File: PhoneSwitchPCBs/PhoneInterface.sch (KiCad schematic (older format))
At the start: 37 parts

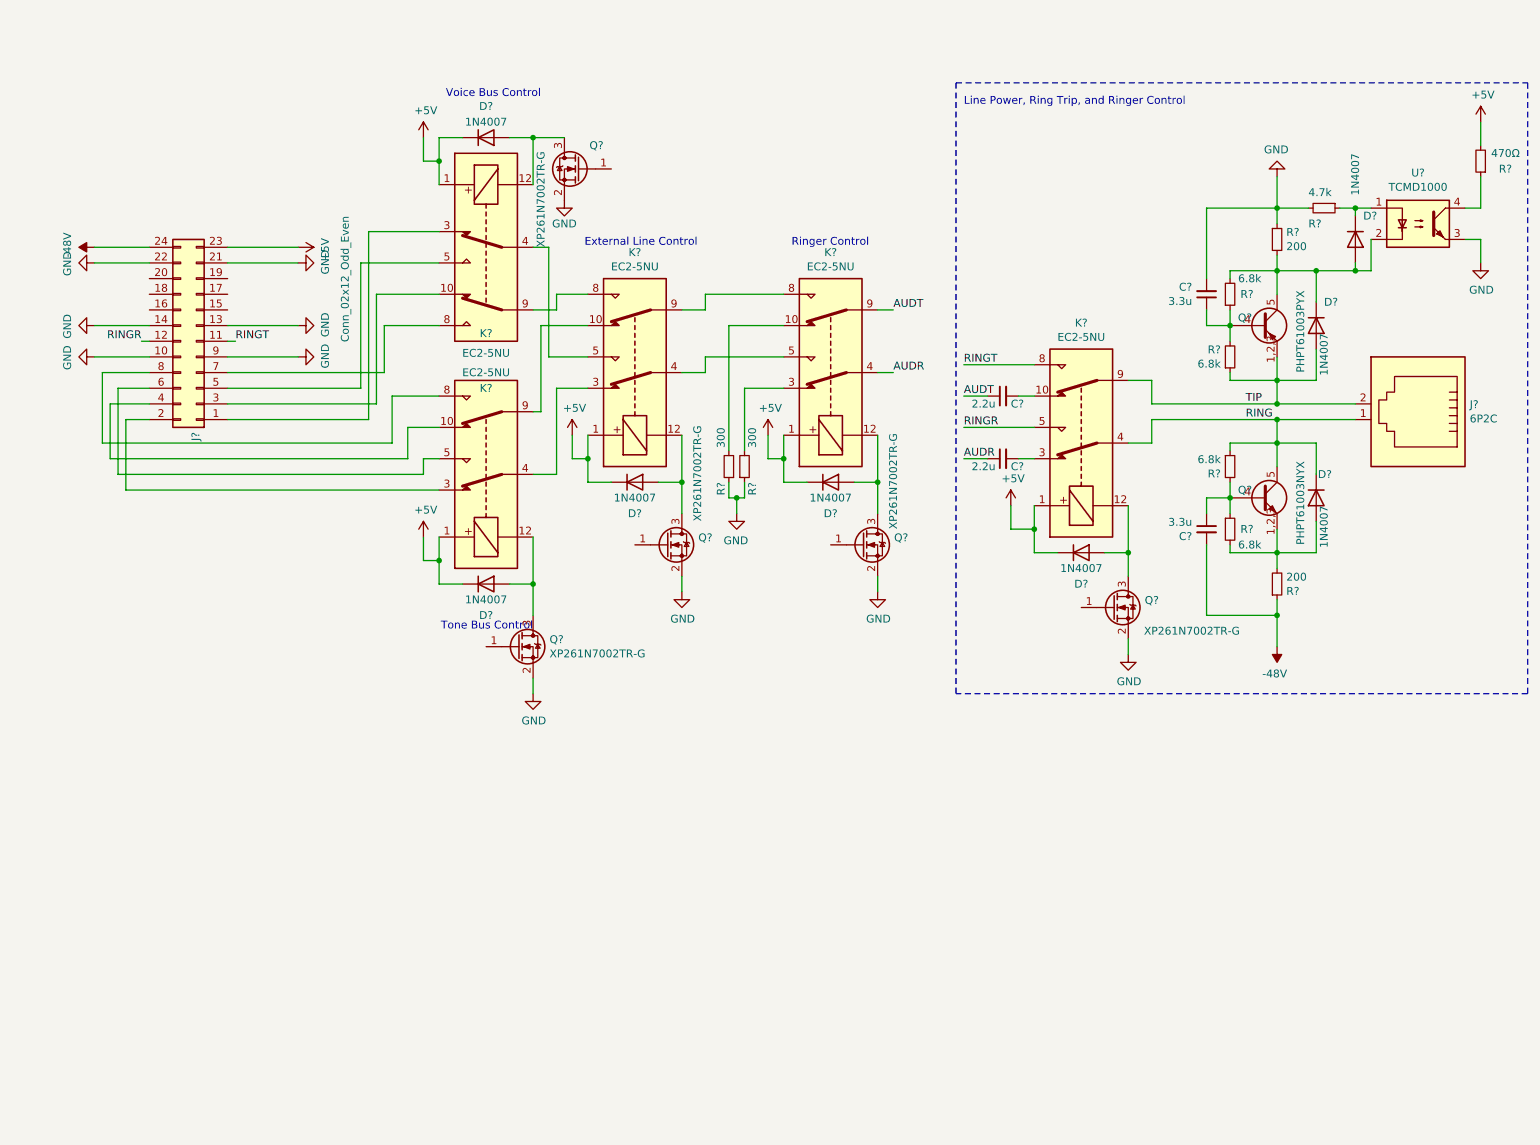
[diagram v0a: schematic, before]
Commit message: Continued work on schematic
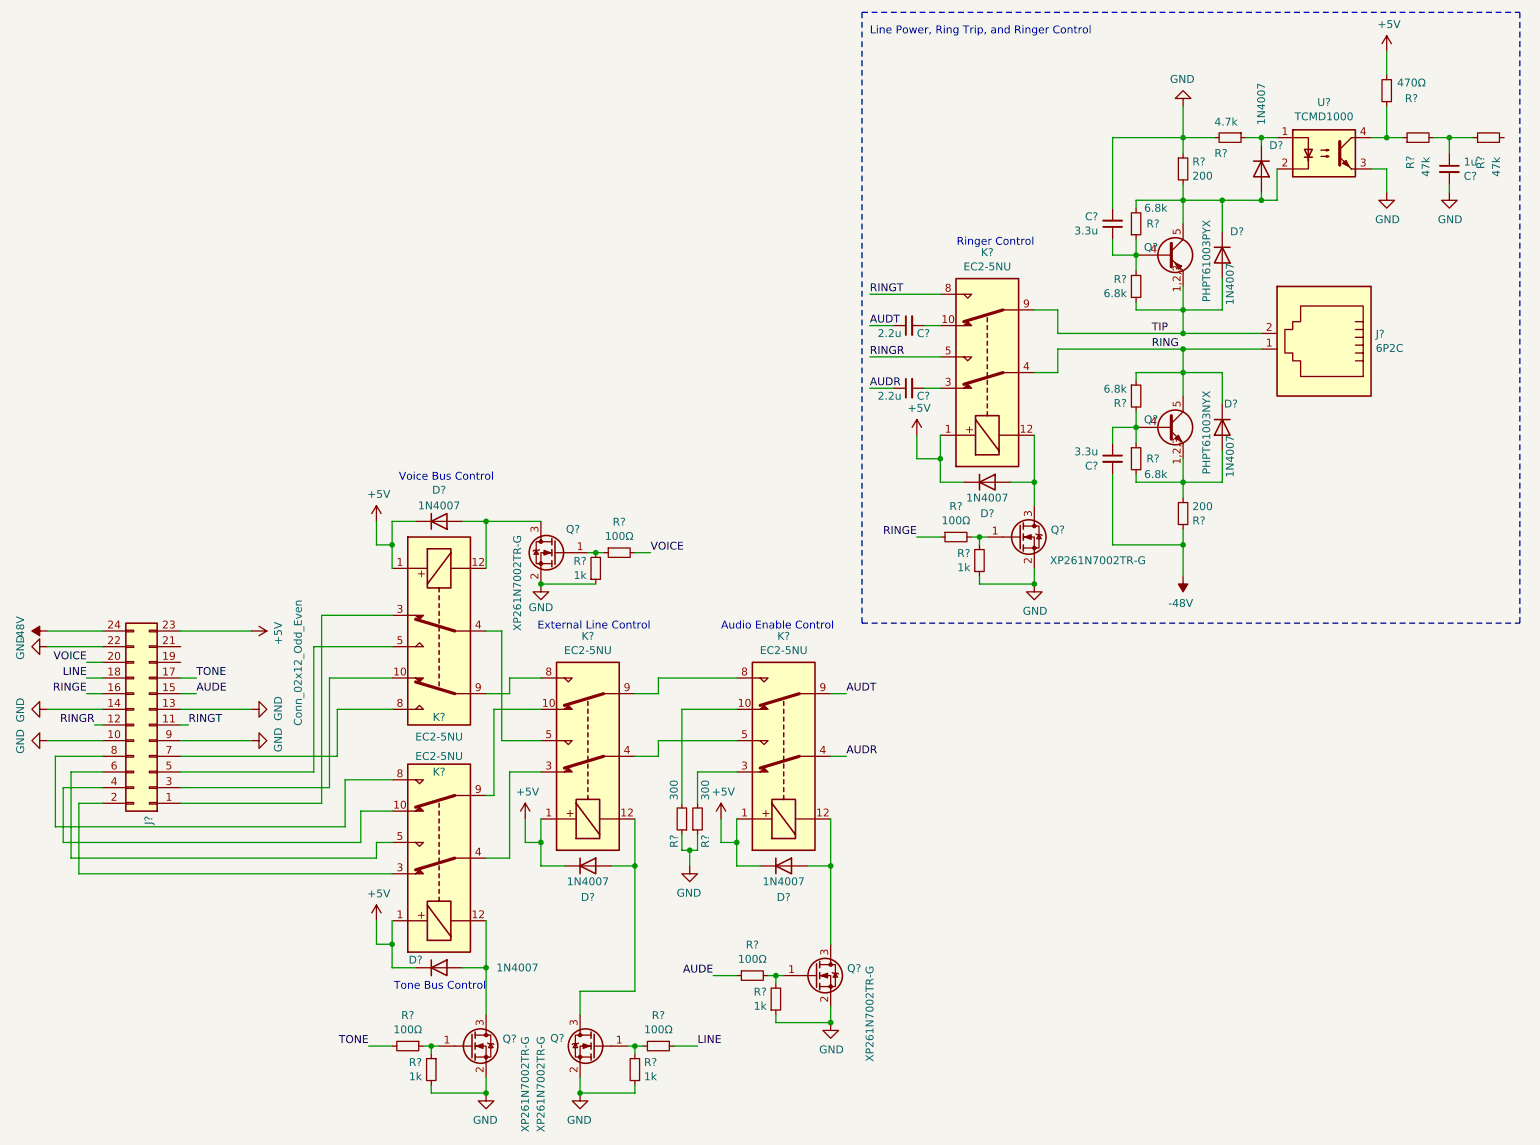
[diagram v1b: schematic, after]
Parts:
- added C?: 1u, symbol Device:C_Small
- added R? (x5): 1k, symbol Device:R_Small
- added R? (x5): 100Ω, symbol Device:R_Small
- added R? (x2): 47k, symbol Device:R_Small
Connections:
- net GND: now also C?.2, R?.1, R?.1, R?.1, R?.1, R?.2; no longer J?.21 (Pin_21)
- net at R?.1, U?.4: now also R?.1
- net at Q?.1 (G): now also R?.2, R?.2 (x3)
- net at Q?.1 (G): now also R?.1, R?.1
- net AUDE: now reaches J?.15 (Pin_15)
- net AUDE: now also R?.1
- net RINGE: now reaches J?.16 (Pin_16)
- net RINGE: now also R?.1
- net TONE: now reaches J?.17 (Pin_17)
- net TONE: now also R?.2
- net LINE: now reaches J?.18 (Pin_18)
- net LINE: now also R?.1
- net VOICE: now reaches J?.20 (Pin_20)
- net VOICE: now also R?.2
- net at Q?.1 (G): now also R?.1, R?.2
- new net: C?.1, R?.1, R?.2
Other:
- note added: "Audio Enable Control"
- moved on the sheet: C?, D?, J?, K?, Q?, R?, U?
